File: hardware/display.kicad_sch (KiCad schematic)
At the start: 5 parts, among them J1 Conn_02x25_Odd_Even_Shielded

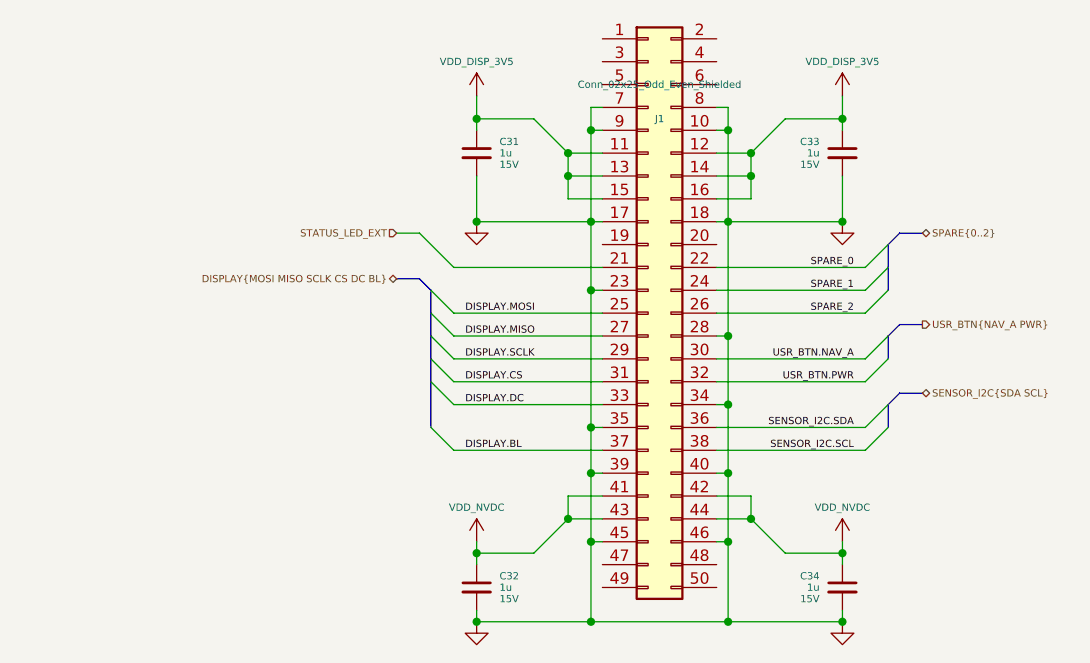
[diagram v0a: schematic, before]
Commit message: Updates
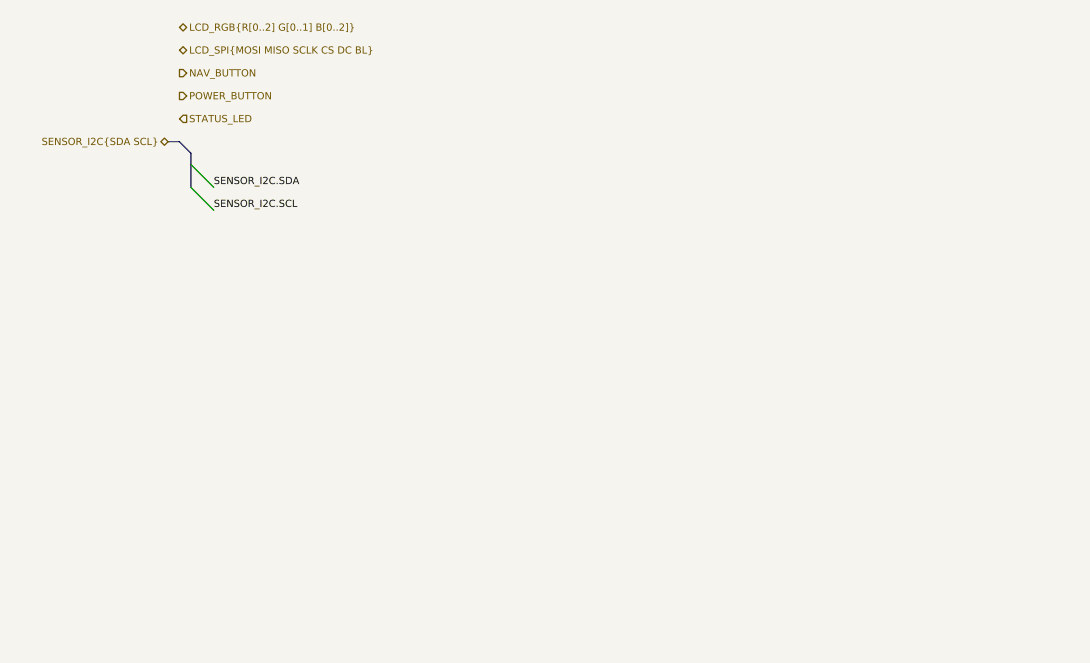
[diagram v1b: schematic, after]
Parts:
- removed C31, C32, C33, C34: 1u, Capacitor_SMD:C_0402_1005Metric, symbol Device:C_Small
- removed J1: Conn_02x25_Odd_Even_Shielded, Connector_Molex:Molex_SlimStack_55560-0501_2x25_P0.50mm_Vertical, symbol Connector_Generic:Conn_02x25_Odd_Even
